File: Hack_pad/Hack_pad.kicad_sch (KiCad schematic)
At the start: 10 parts, among them SW1 SW_Push, SW2 SW_Push, SW3 SW_Push, SW4 SW_Push, SW5 RotaryEncoder_Switch, U1 XIAO-RP2040-DIP

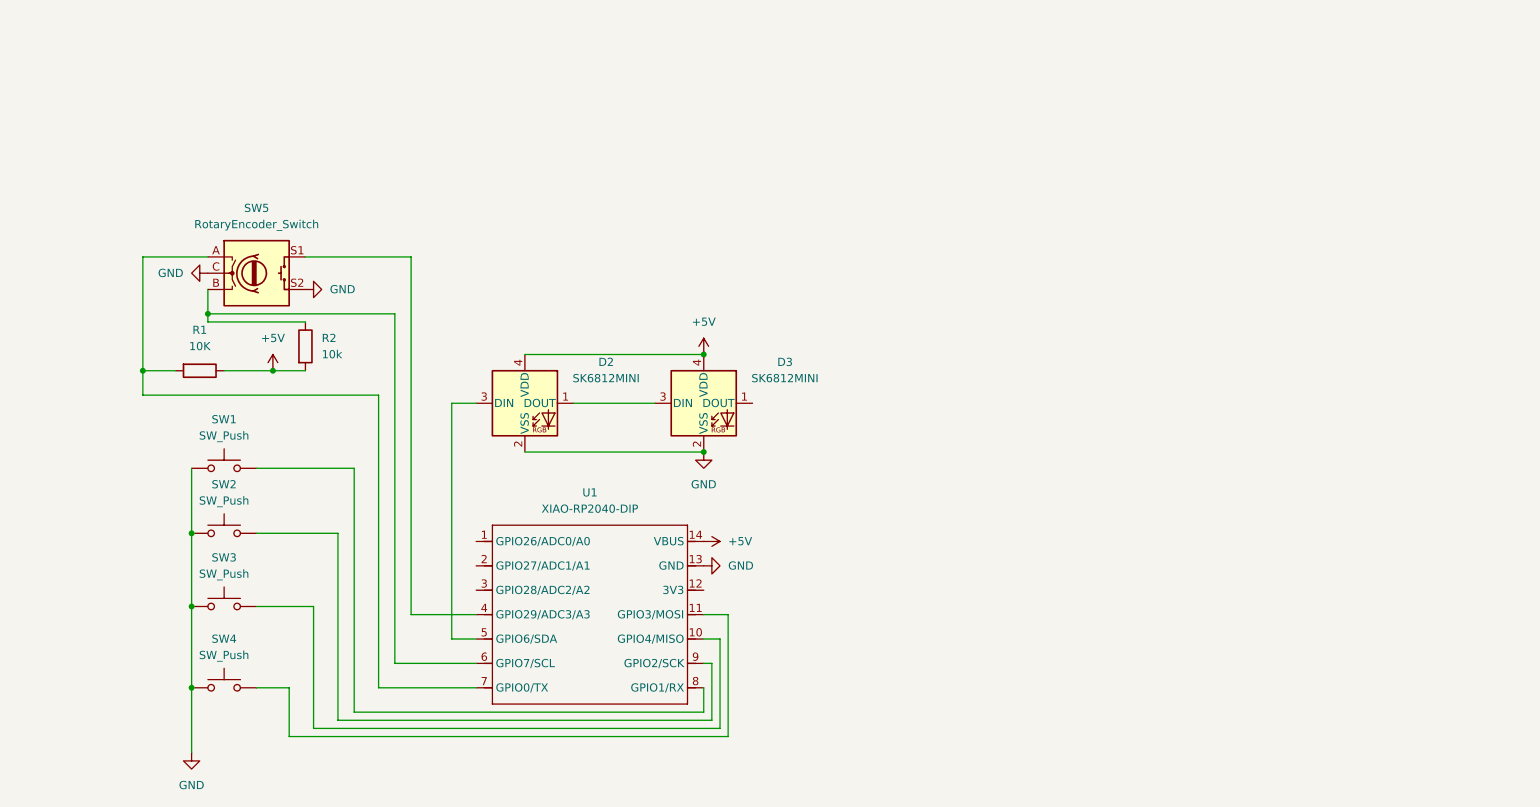
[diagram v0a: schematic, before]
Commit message: update
recrated
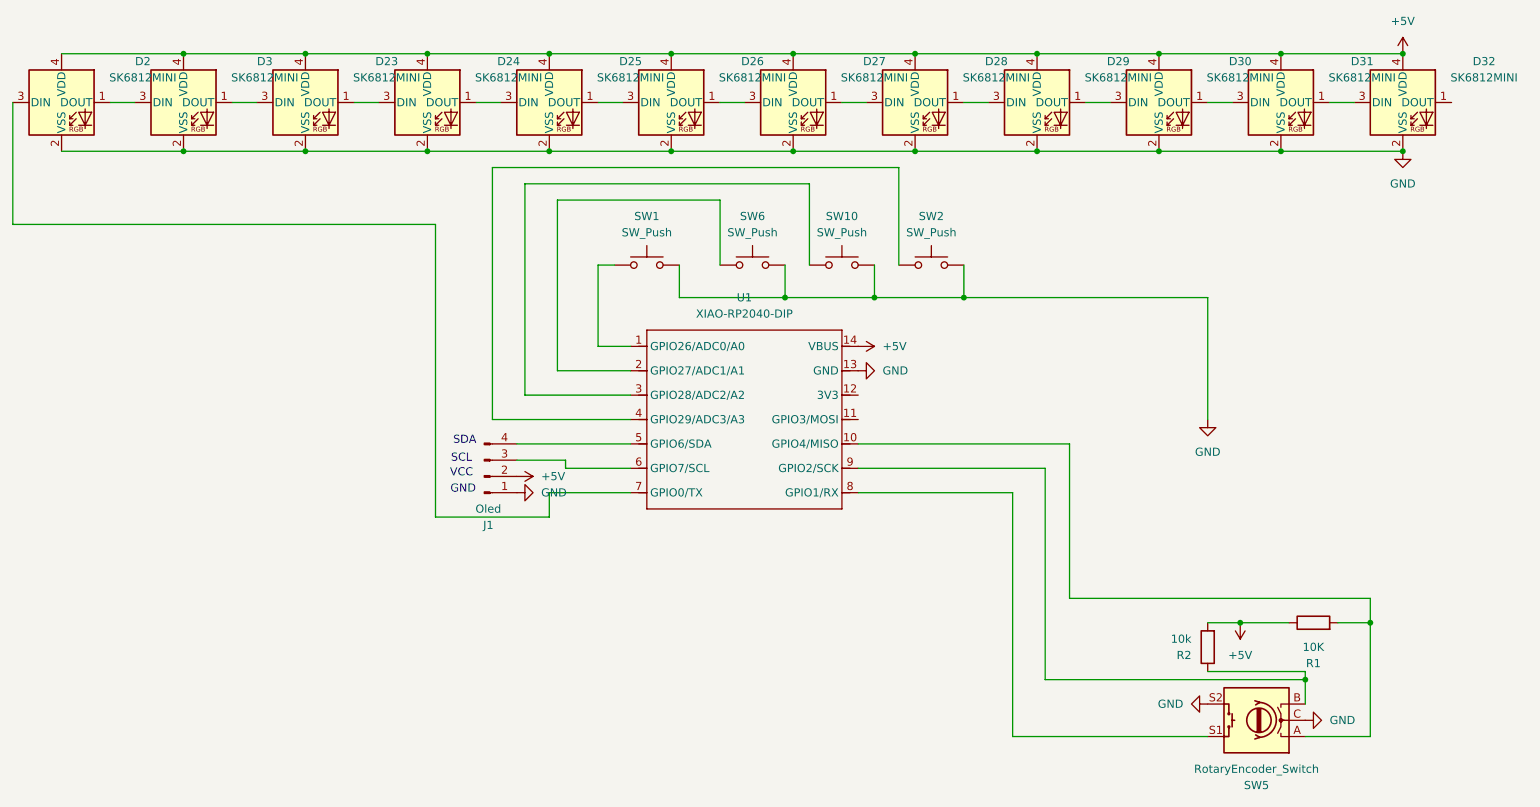
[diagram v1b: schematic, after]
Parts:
- removed SW3, SW4: SW_Push, Button_Switch_Keyboard:SW_Cherry_MX_1.00u_PCB, symbol Switch:SW_Push
- added D23, D24, D25, D26, D27, D28, D29, D30, D31, D32: SK6812MINI, LED_SMD:LED_SK6812MINI_PLCC4_3.5x3.5mm_P1.75mm, symbol LED:SK6812MINI
- added J1: Oled, oled:SSD1306-0.91-OLED-4pin-128x32, symbol Connector:Conn_01x04_Pin
- added SW10, SW6: SW_Push, Button_Switch_Keyboard:SW_Cherry_MX_1.00u_PCB, symbol Switch:SW_Push
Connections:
- net +5V: now also D23.4 (VDD), D24.4 (VDD), D25.4 (VDD), D26.4 (VDD), D27.4 (VDD), D28.4 (VDD), D29.4 (VDD), D30.4 (VDD), D31.4 (VDD), D32.4 (VDD), J1.2 (Pin_2)
- net GND: now also SW1.2, SW2.2, D23.2 (VSS), D24.2 (VSS), D25.2 (VSS), D26.2 (VSS), D27.2 (VSS), D28.2 (VSS), D29.2 (VSS), D30.2 (VSS), D31.2 (VSS), D32.2 (VSS), J1.1 (Pin_1), SW10.2, SW6.2; no longer SW1.1, SW2.1
- net at U1.8 (GPIO1/RX): now also SW5.S1; no longer SW1.2
- net at U1.9 (GPIO2/SCK): now also R2.1, SW5.B; no longer SW2.2
- net at R1.2, SW5.A: now also U1.10 (GPIO4/MISO); no longer U1.7 (GPIO0/TX)
- net at U1.4 (GPIO29/ADC3/A3): now also SW2.1; no longer SW5.S1
- net at D3.1 (DOUT): now also D23.3 (DIN)
- net at U1.5 (GPIO6/SDA): now also J1.4 (Pin_4); no longer D2.3 (DIN)
- net at U1.1 (GPIO26/ADC0/A0): now also SW1.1
- net at U1.2 (GPIO27/ADC1/A1): now also SW6.1
- net at U1.3 (GPIO28/ADC2/A2): now also SW10.1
- new net: J1.3 (Pin_3), U1.6 (GPIO7/SCL)
- new net: D2.3 (DIN), U1.7 (GPIO0/TX)
- new net: D24.1 (DOUT), D25.3 (DIN)
- new net: D23.1 (DOUT), D24.3 (DIN)
- new net: D25.1 (DOUT), D26.3 (DIN)
- new net: D29.1 (DOUT), D30.3 (DIN)
- new net: D28.1 (DOUT), D29.3 (DIN)
- new net: D26.1 (DOUT), D27.3 (DIN)
- new net: D31.1 (DOUT), D32.3 (DIN)
- new net: D30.1 (DOUT), D31.3 (DIN)
- new net: D27.1 (DOUT), D28.3 (DIN)
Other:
- note added: "GND"
- note added: "SCL"
- note added: "SDA"
- note added: "VCC"
- moved on the sheet: D2, D3, R1, R2, SW1, SW2, SW5
